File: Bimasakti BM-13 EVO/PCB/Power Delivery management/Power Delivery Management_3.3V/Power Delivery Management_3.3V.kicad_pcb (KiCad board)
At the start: 2 copper layers, 35 x 43 mm, 31 parts, among them J1 +12V In, J2 3.3V

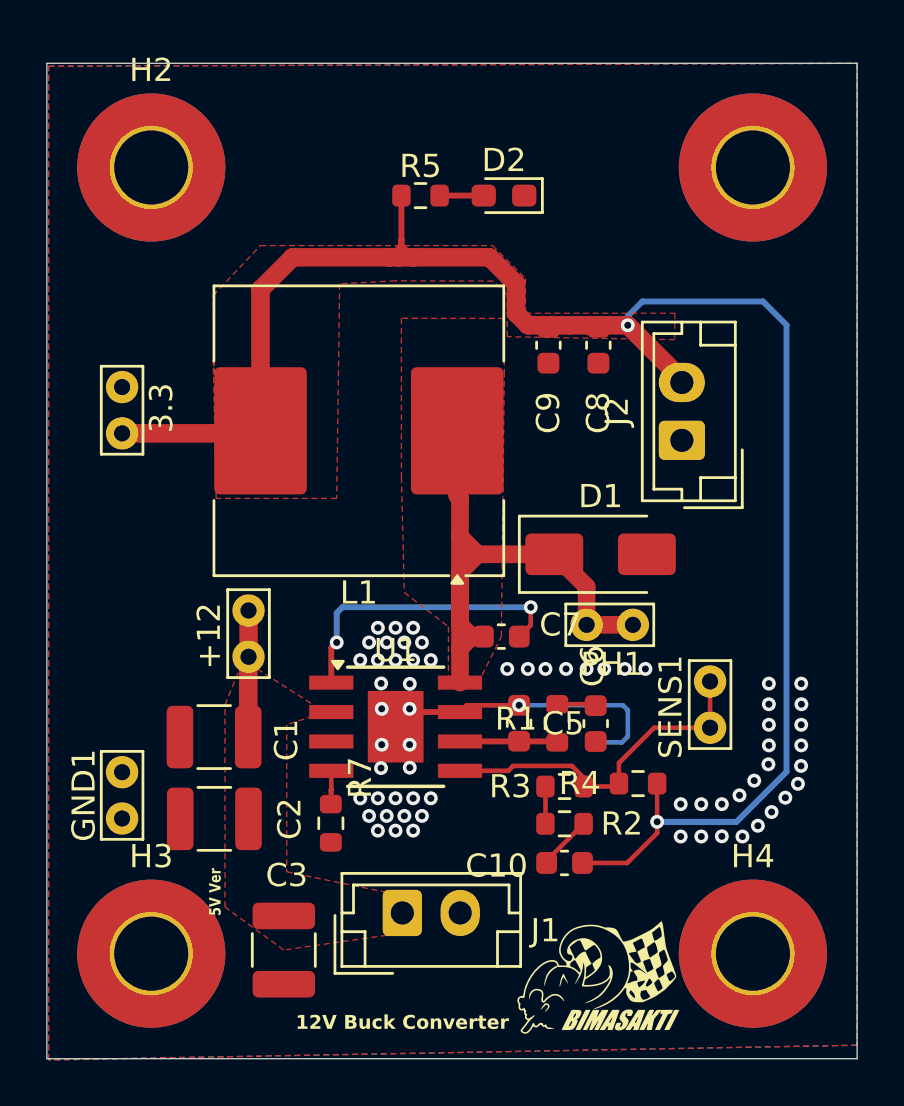
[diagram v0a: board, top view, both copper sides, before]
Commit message: cicil assembly
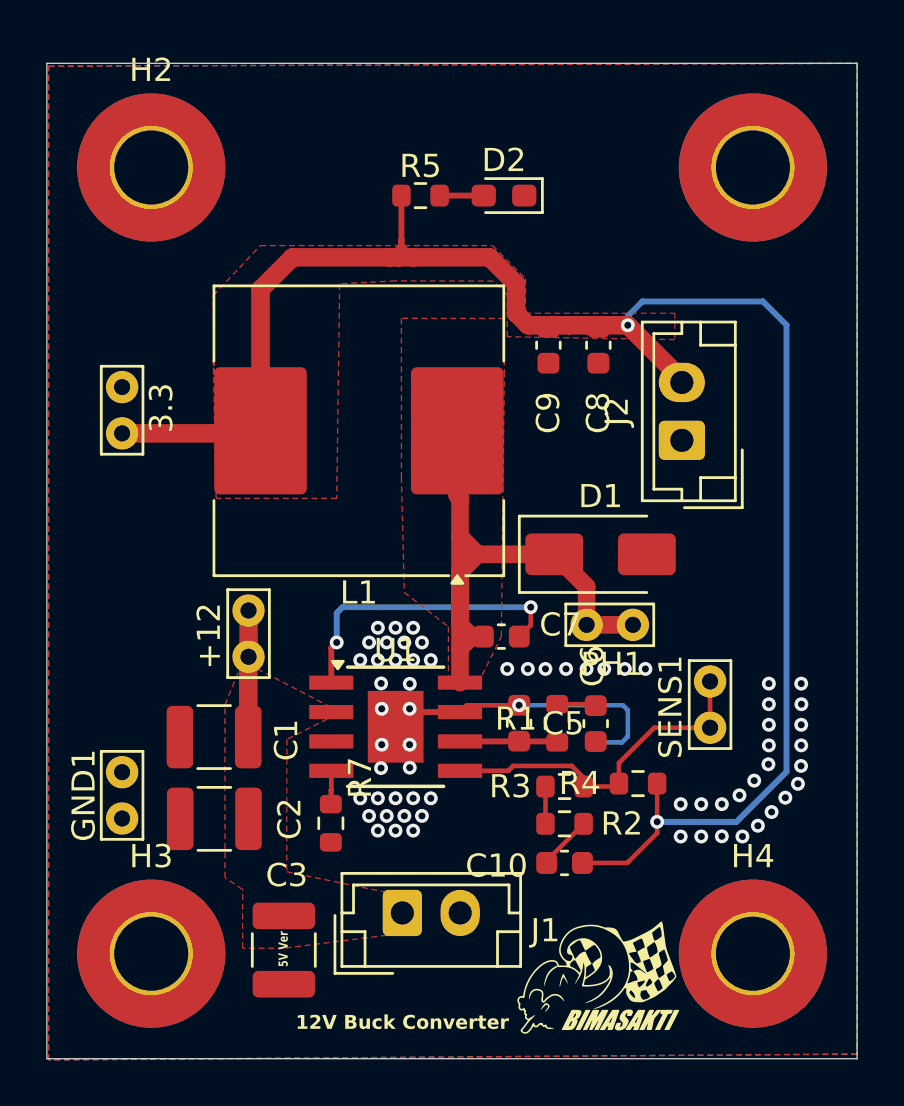
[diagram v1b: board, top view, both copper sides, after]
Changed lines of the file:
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@@
 	)
 	(gr_text "5V Ver\n"
-		(at 48.387 66.167 90)
+		(at 51.27238 68.373138 90)
 		(layer "F.SilkS")
 		(effects
 			(font
-				(size 0.5 0.4)
-				(thickness 0.08)
+				(size 0.4 0.3)
+				(thickness 0.06)
 				(bold yes)
 			)
@@
 		(polygon
 			(pts
-				(xy 48.514 65.786) (xy 48.514 57.046385) (xy 49.149 55.499) (xy 49.911 55.499) (xy 49.911 55.499)
-				(xy 52.324 57.046385) (xy 52.324 57.531) (xy 51.181 57.912) (xy 51.181 64.262) (xy 55.499 65.151)
-				(xy 55.499 67.004252) (xy 51.054 67.642)
+				(xy 49.276 67.564) (xy 49.276 65.024) (xy 48.514 64.516) (xy 48.514 57.046385) (xy 49.149 55.499)
+				(xy 49.911 55.499) (xy 52.94547 57.077206) (xy 52.936392 57.658173) (xy 51.184761 58.542893) (xy 51.181 64.262)
+				(xy 55.499 65.151) (xy 55.499 67.004252) (xy 51.054 67.564)
 			)
 		)
@@
 		(layers "F.Cu" "B.Cu")
 		(hatch edge 0.5)
-		(connect_pads yes
+		(connect_pads
 			(clearance 0.381)
 		)
@@
 		(polygon
 			(pts
-				(xy 40.894 29.464) (xy 75.819 29.337) (xy 75.819 71.755) (xy 40.894 72.39)
+				(xy 40.894 29.464) (xy 75.819 29.337) (xy 75.819 72.136) (xy 40.894 72.39)
 			)
 		)
